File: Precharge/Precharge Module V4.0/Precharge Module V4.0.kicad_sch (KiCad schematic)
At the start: 22 parts, among them J1 PH1-10-UA, Q1 SS8550, U1 NE555D, U2 IRLML2060TRPBF, U3 IRLML2060TRPBF, U4 IRLML2060TRPBF, U5 PMV160UP

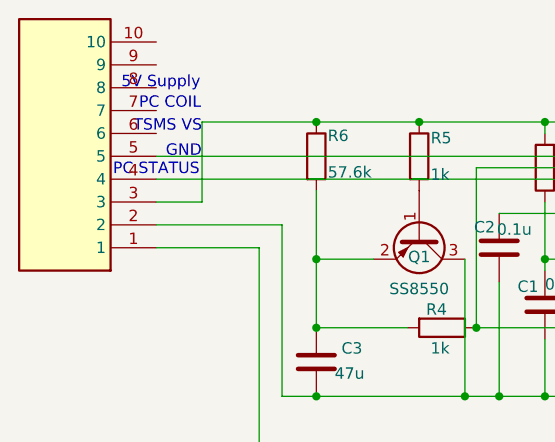
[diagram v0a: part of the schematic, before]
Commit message: Renaming stuff on boards that was wrong
RTDS schematic was totally totally wrong with the pins compared to the PCB
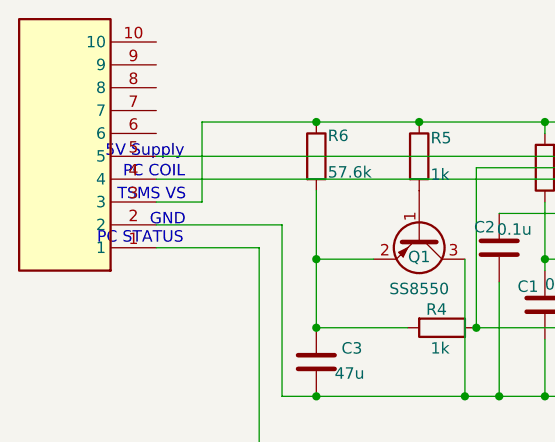
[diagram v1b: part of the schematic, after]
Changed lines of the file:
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@@
 (kicad_sch
-	(version 20231120)
+	(version 20250114)
 	(generator "eeschema")
-	(generator_version "8.0")
+	(generator_version "9.0")
 	(paper "A4")
+	(text "GND"
+		(exclude_from_sim no)
+		(at 33.02 36.322 0)
+		(effects
+			(font
+				(size 1.27 1.27)
+			)
+		)
+	)
+	(text "PC COIL"
+		(exclude_from_sim no)
+		(at 31.496 30.988 0)
+		(effects
+			(font
+				(size 1.27 1.27)
+			)
+		)
+	)
+	(text "TSMS VS"
+		(exclude_from_sim no)
+		(at 31.242 33.528 0)
+		(effects
+			(font
+				(size 1.27 1.27)
+			)
+		)
+	)
+	(text "PC STATUS"
+		(exclude_from_sim no)
+		(at 29.972 38.354 0)
+		(effects
+			(font
+				(size 1.27 1.27)
+			)
+		)
+	)
+	(text "5V Supply"
+		(exclude_from_sim no)
+		(at 30.48 28.702 0)
+		(effects
+			(font
+				(size 1.27 1.27)
+			)
+		)
+	)
 	(junction
 		(at 109.22 30.48)
@@
 			(width 0)
 			(type default)
-		)
-	)
-	(text "GND"
-		(exclude_from_sim no)
-		(at 34.798 28.702 0)
-		(effects
-			(font
-				(size 1.27 1.27)
-			)
-		)
-	)
-	(text "PC COIL"
-		(exclude_from_sim no)
-		(at 33.274 23.368 0)
-		(effects
-			(font
-				(size 1.27 1.27)
-			)
-		)
-	)
-	(text "TSMS VS"
-		(exclude_from_sim no)
-		(at 33.02 25.908 0)
-		(effects
-			(font
-				(size 1.27 1.27)
-			)
-		)
-	)
-	(text "PC STATUS"
-		(exclude_from_sim no)
-		(at 31.75 30.734 0)
-		(effects
-			(font
-				(size 1.27 1.27)
-			)
-		)
-	)
-	(text "5V Supply"
-		(exclude_from_sim no)
-		(at 32.258 21.082 0)
-		(effects
-			(font
-				(size 1.27 1.27)
-			)
 		)
 	)
@@
 		)
 	)
+	(embedded_fonts no)
 )
